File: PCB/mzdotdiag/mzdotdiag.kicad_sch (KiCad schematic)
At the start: 1 part, among them J1 Conn_01x25

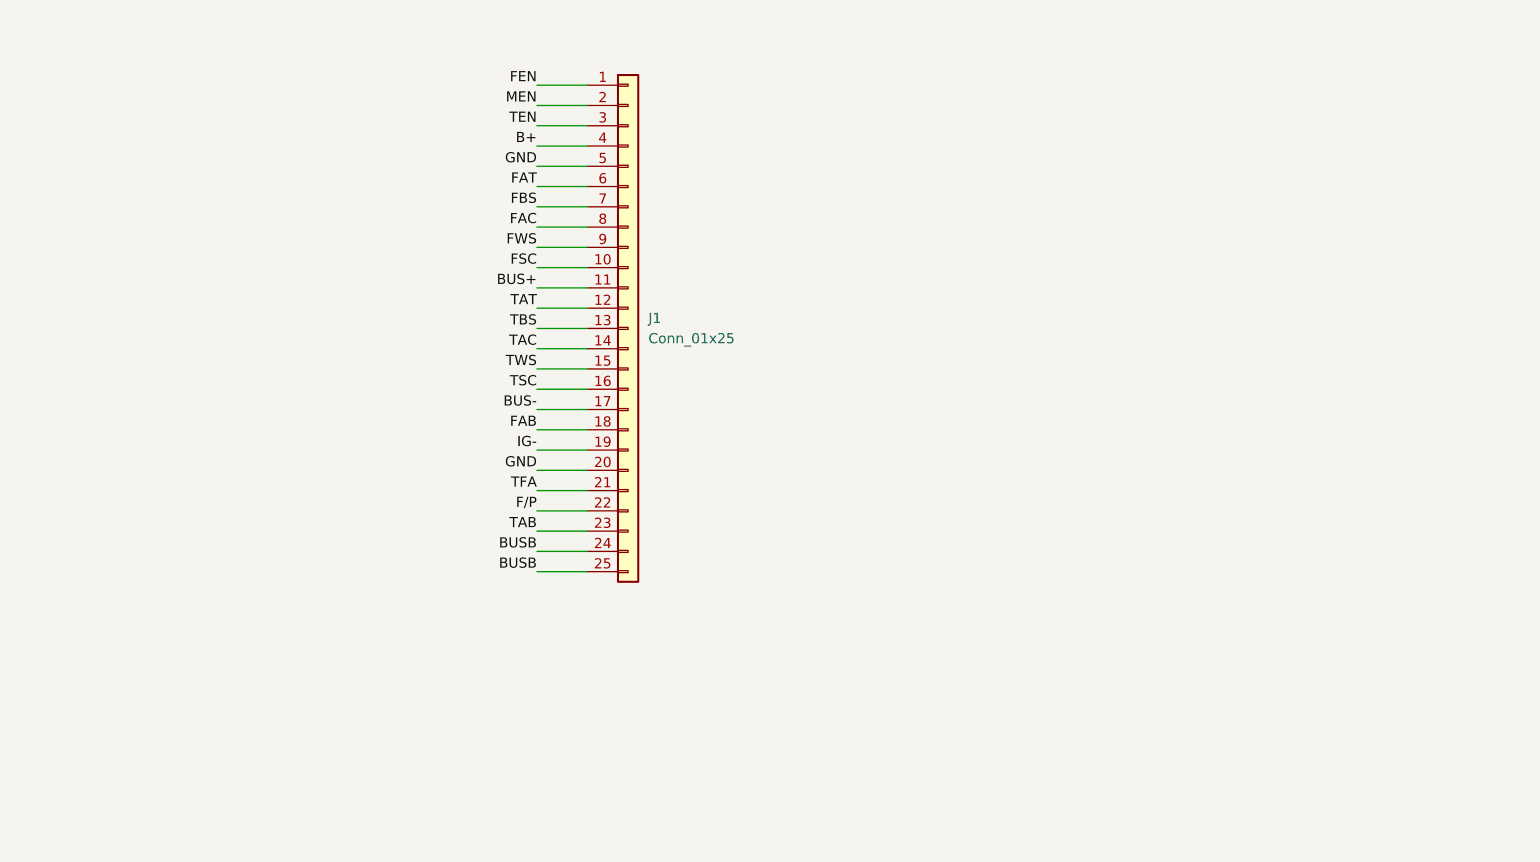
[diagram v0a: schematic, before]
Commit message: advancements in schematic
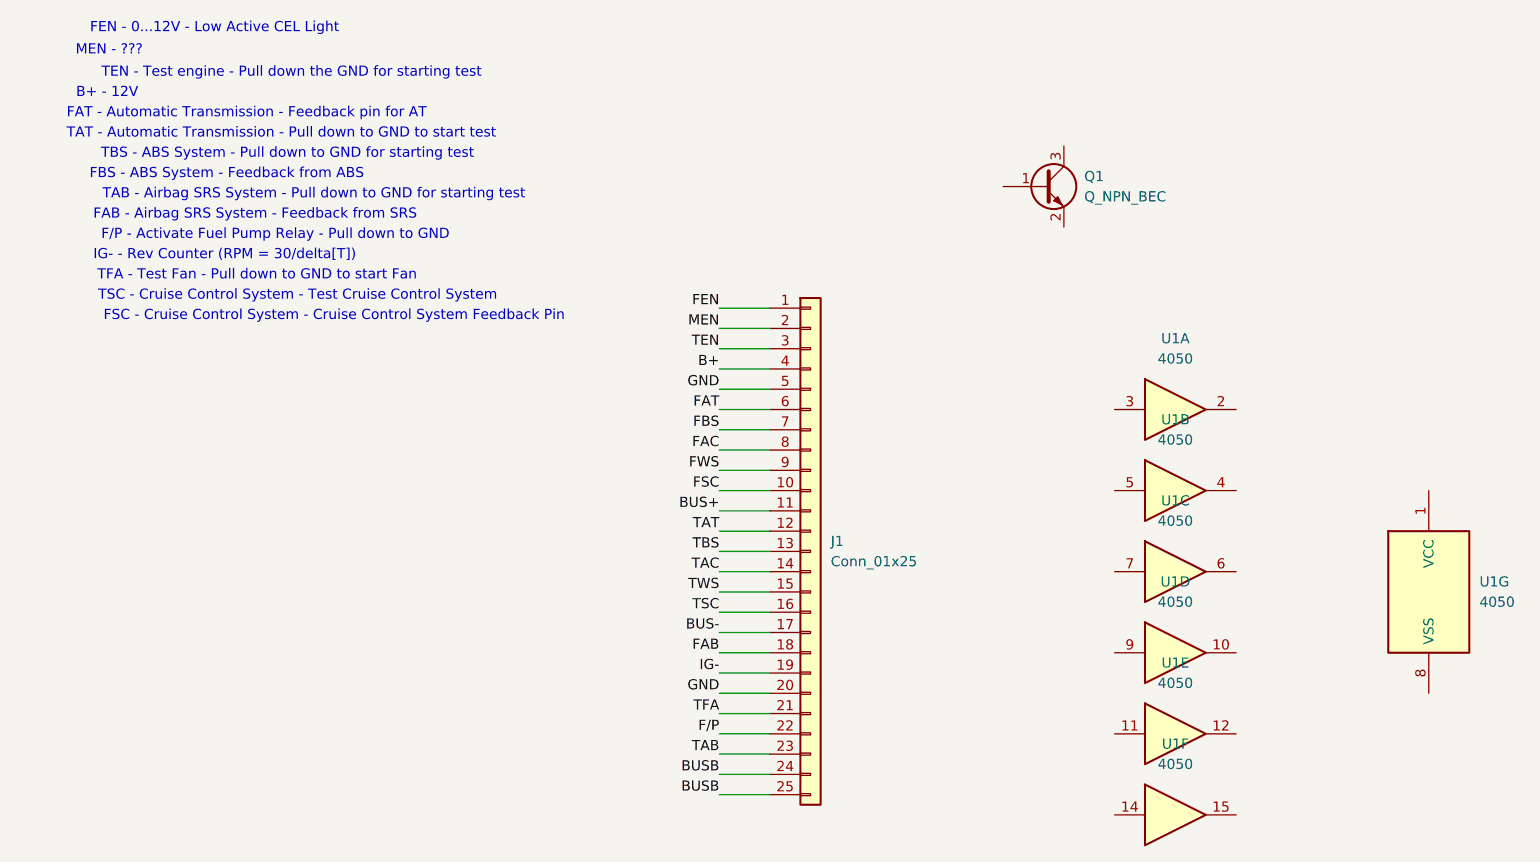
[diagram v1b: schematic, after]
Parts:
- added Q1: Q_NPN_BEC, symbol Device:Q_NPN_BEC
- added U1: 4050, symbol 4xxx:4050
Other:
- note added: "B+ - 12V"
- note added: "F/P - Activate Fuel Pump Relay - Pull down to GND"
- note added: "FAB - Airbag SRS System - Feedback from SRS"
- note added: "FAT - Automatic Transmission - Feedback pin for AT"
- note added: "FBS - ABS System - Feedback from ABS"
- note added: "FEN - 0...12V - Low Active CEL Light"
- note added: "FSC - Cruise Control System - Cruise Control System Feedback Pin"
- note added: "IG- - Rev Counter (RPM = 30/delta[T])"
- note added: "MEN - ???"
- note added: "TAB - Airbag SRS System - Pull down to GND for starting test"
- note added: "TAT - Automatic Transmission - Pull down to GND to start test"
- note added: "TBS - ABS System - Pull down to GND for starting test"
- note added: "TEN - Test engine - Pull down the GND for starting test"
- note added: "TFA - Test Fan - Pull down to GND to start Fan"
- note added: "TSC - Cruise Control System - Test Cruise Control System"
- moved on the sheet: J1
